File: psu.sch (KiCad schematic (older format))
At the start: 17 parts, among them U7 LM2596S-ADJ, U8 LM2596S-ADJ

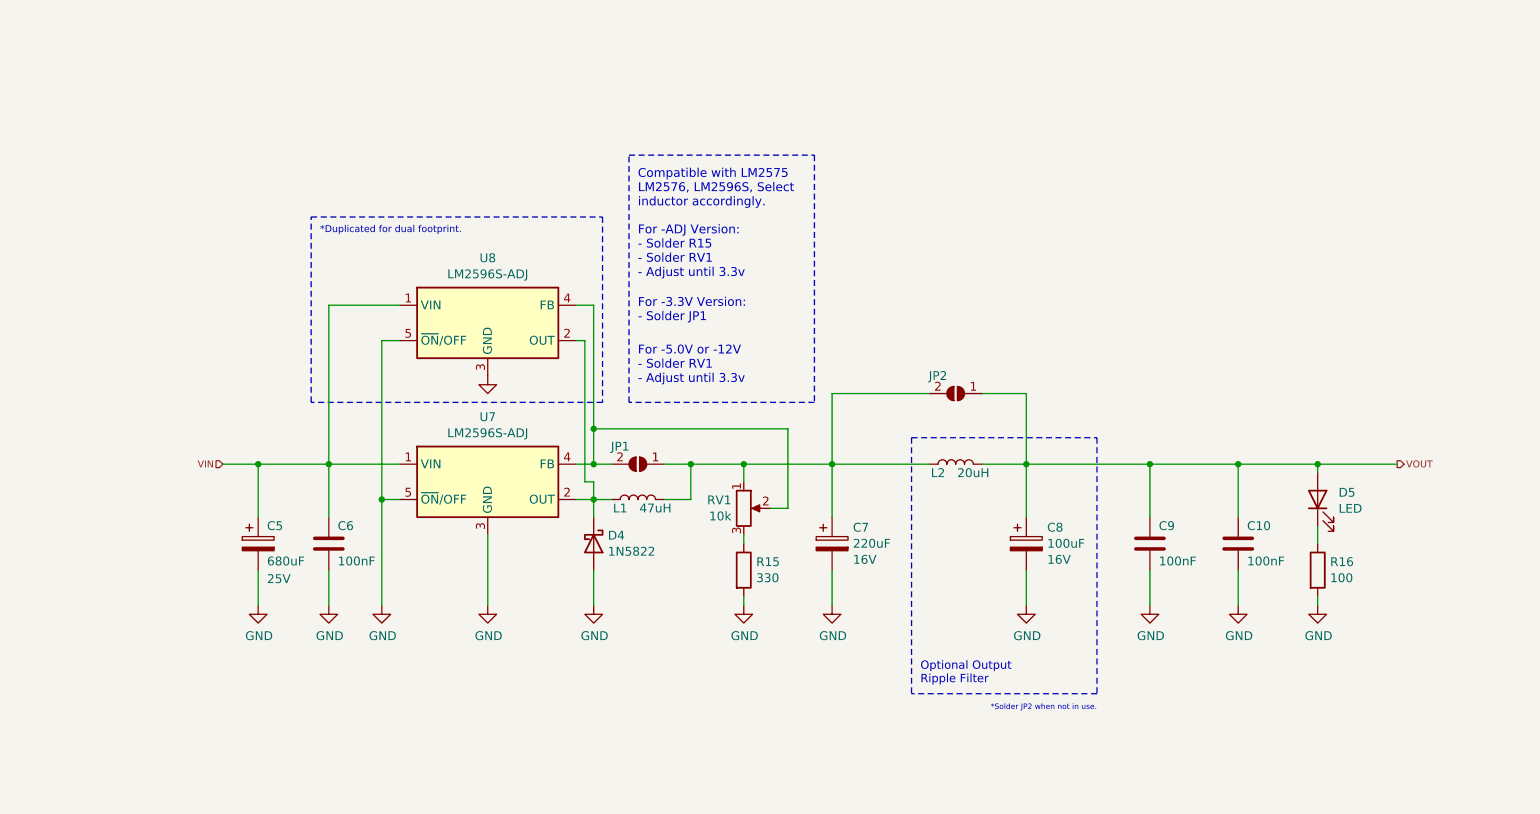
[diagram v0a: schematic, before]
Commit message: Several changes.
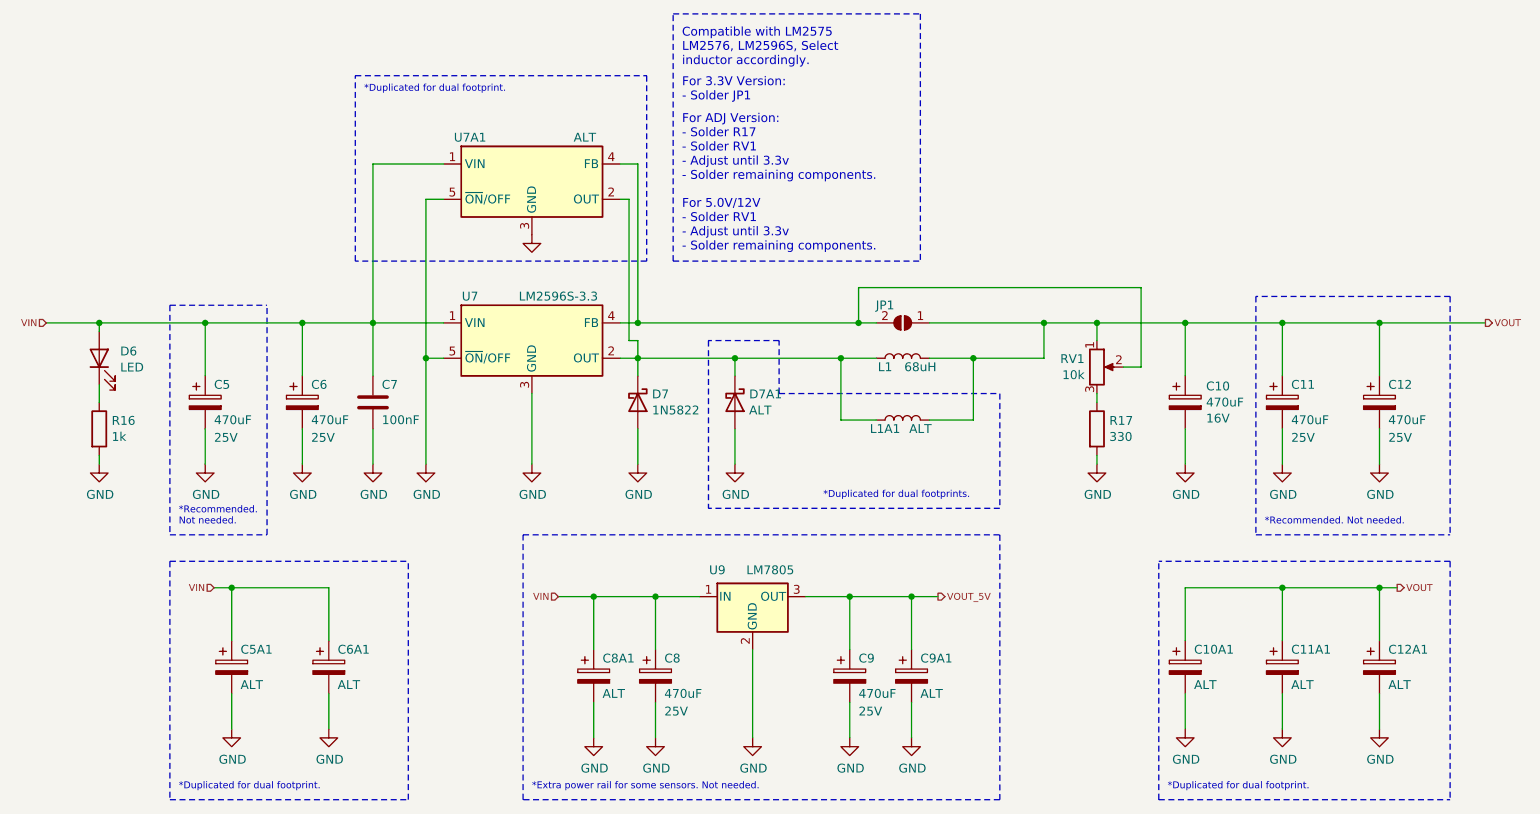
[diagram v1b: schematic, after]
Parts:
- removed C10, C9: 100nF, Capacitor_SMD:C_1206_3216Metric_Pad1.33x1.80mm_HandSolder, symbol Device:C
- removed JP2: SolderJumper_2_Open, symbol Jumper:SolderJumper_2_Open
- removed L2: 20uH, symbol Device:L
- removed U7, U8: LM2596S-ADJ, Package_TO_SOT_SMD:TO-263-5_TabPin3, symbol Regulator_Switching:LM2596S-ADJ
- added C10A1, C11A1, C12A1, C5A1, C6A1, C8A1, C9A1: ALT, symbol Device:CP
- added C11, C12, C5, C9: 470uF, symbol Device:CP
- added D7A1: ALT, Diode_THT:D_DO-201_P12.70mm_Horizontal, symbol Diode:1N5822
- added L1A1: ALT, symbol Device:L
- added U7: LM2596S-3.3, Package_TO_SOT_SMD:TO-263-5_TabPin3, symbol Regulator_Switching:LM2596S-3.3
- added U7A1: ALT, Package_TO_SOT_THT:TO-220-5_Vertical, symbol Regulator_Switching:LM2596S-3.3
- added U9: LM7805, symbol Regulator_Linear:L7805
- C10: renamed from C7; value 220uF -> 470uF
- C6: renamed from C5; value 680uF -> 470uF
- C8: value 100uF -> 470uF; Fitted (none) -> No; Voltage 16V -> 25V
- L1: value 47uH -> 68uH
- R16: value 100 -> 1k
- R17: renamed from R15; Fitted (none) -> No
- RV1: Fitted (none) -> No
- renumbered C6 to C7, D5 to D6, D4 to D7
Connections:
- net GND: now also C10A1.2, C11.2, C11A1.2, C12.2, C12A1.2, C5.2, C5A1.2, C6A1.2, C8A1.2, C9.2, C9A1.2, D7A1.2 (A), U7.3 (GND), U7.5 (~ON~/OFF), U7A1.3 (GND), U7A1.5 (~ON~/OFF), U9.2 (GND)
- net VIN: now also C8.1, D6.2 (A), C5.1, C5A1.1, C6A1.1, C8A1.1, U7.1 (VIN), U7A1.1 (VIN), U9.1 (IN)
- net VOUT: now also C10.1, JP1.1 (A), L1.2, RV1.1, C10A1.1, C11.1, C11A1.1, C12.1, C12A1.1, L1A1.2; no longer C8.1, D6.2 (A)
- net at D7.1 (K), L1.1: now also D7A1.1 (K), L1A1.1, U7.2 (OUT), U7A1.2 (OUT)
- net at JP1.2 (B), RV1.2: now also U7.4 (FB), U7A1.4 (FB)
- new net VOUT_5V: C9.1, C9A1.1, U9.3 (OUT)
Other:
- note added: "*Duplicated for dual footprints."
- note added: "*Extra power rail for some sensors. Not needed."
- note added: "*Recommended. Not needed."
- note added: "*Recommended. \nNot needed."
- note added: "For 3.3V Version:\n- Solder JP1"
- note added: "For 5.0V/12V\n- Solder RV1\n- Adjust until 3.3v\n- Solder remaining components."
- note added: "For ADJ Version:\n- Solder R17\n- Solder RV1\n- Adjust until 3.3v\n- Solder remaining components."
- note removed: "*Solder JP2 when not in use."
- note removed: "For -3.3V Version:\n- Solder JP1"
- note removed: "For -5.0V or -12V\n- Solder RV1\n- Adjust until 3.3v"
- note removed: "For -ADJ Version:\n- Solder R15\n- Solder RV1\n- Adjust until 3.3v"
- note removed: "Optional Output\nRipple Filter"
- moved on the sheet: C10, C6, C7, D6, D7, JP1, L1, R16, R17, RV1
